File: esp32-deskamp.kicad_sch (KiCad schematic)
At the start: 29 parts, among them J1 INPUT 00, J10 ADDITIONAL GPIO, J2 INPUT 01, J3 MUTE, J4 SLEEP, J5 PRE OUT, J6 LFE OUT, J7 INPUT SELECT, J8 MOTOR, J9 12V IN, K1 INPUT 00, K2 INPUT 01, K3 AMP MUTE, K4 AMP SLEEP, U1 ESP32 D1 MINI, U2 TSR 1-2433, U3 L9110, U4 ULN2003A

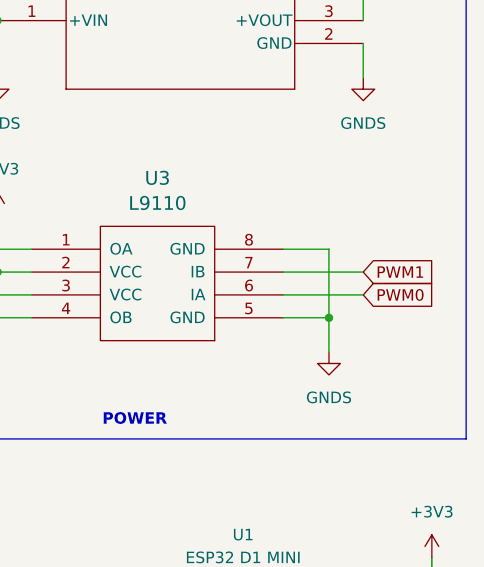
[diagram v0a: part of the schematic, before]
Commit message: Moar routing
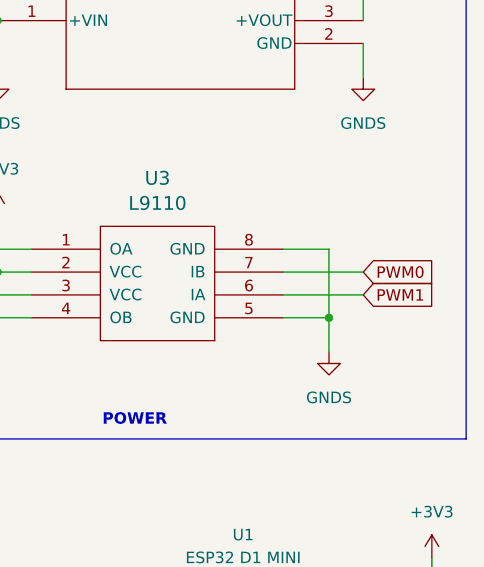
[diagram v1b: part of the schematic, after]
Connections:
- net PWM0: now also U3.7 (IB); no longer U3.6 (IA)
- net PWM1: now also U3.6 (IA); no longer U3.7 (IB)
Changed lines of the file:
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@@
-		)
-	)
-	(global_label "PWM0"
-		(shape input)
-		(at 267.97 59.69 0)
-		(fields_autoplaced yes)
-		(effects
-			(font
-				(size 1.27 1.27)
-			)
-			(justify left)
-		)
-		(property "Intersheetrefs" "${INTERSHEET_REFS}"
-			(at 276.3375 59.69 0)
-			(effects
-				(font
-					(size 1.27 1.27)
-				)
-				(justify left)
-				(hide yes)
-			)
 		)
 	)
@@
 		(property "Intersheetrefs" "${INTERSHEET_REFS}"
 			(at 89.3451 49.53 0)
-			(effects
-				(font
-					(size 1.27 1.27)
-				)
-				(justify left)
-				(hide yes)
-			)
-		)
-	)
-	(global_label "PWM1"
-		(shape input)
-		(at 267.97 57.15 0)
-		(fields_autoplaced yes)
-		(effects
-			(font
-				(size 1.27 1.27)
-			)
-			(justify left)
-		)
-		(property "Intersheetrefs" "${INTERSHEET_REFS}"
-			(at 276.3375 57.15 0)
 			(effects
 				(font
@@
 		)
 	)
+	(global_label "PWM0"
+		(shape input)
+		(at 267.97 57.15 0)
+		(fields_autoplaced yes)
+		(effects
+			(font
+				(size 1.27 1.27)
+			)
+			(justify left)
+		)
+		(property "Intersheetrefs" "${INTERSHEET_REFS}"
+			(at 276.3375 57.15 0)
+			(effects
+				(font
+					(size 1.27 1.27)
+				)
+				(justify left)
+				(hide yes)
+			)
+		)
+	)
 	(global_label "Select0"
 		(shape input)
@@
 				(hide yes)
 			)
+		)
+	)
+	(global_label "PWM1"
+		(shape input)
+		(at 267.97 59.69 0)
+		(fields_autoplaced yes)
+		(effects
+			(font
+				(size 1.27 1.27)
+			)
+			(justify left)
+		)
+		(property "Intersheetrefs" "${INTERSHEET_REFS}"
+			(at 276.3375 59.69 0)
+			(effects
+				(font
+					(size 1.27 1.27)
+				)
+				(justify left)
+				(hide yes)
+			)

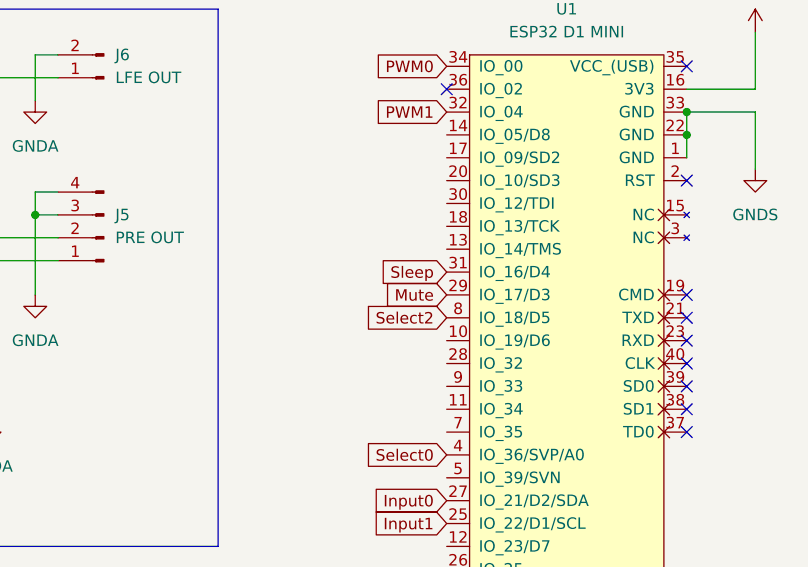
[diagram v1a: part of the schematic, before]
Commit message: Enough for tonight, routed relay control board
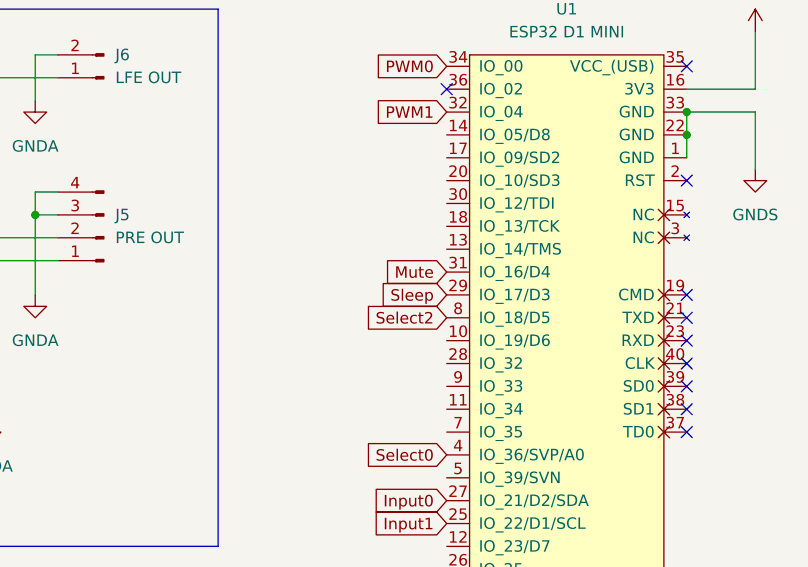
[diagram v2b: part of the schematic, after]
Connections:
- net Mute: now also U1.31 (IO_16/D4); no longer U1.29 (IO_17/D3)
- net Sleep: now also U1.29 (IO_17/D3); no longer U1.31 (IO_16/D4)

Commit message: Moar layout
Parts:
- R7, R8, R9: footprint Resistor_SMD:R_0805_2012Metric_Pad1.20x1.40mm_HandSolder -> Resistor_THT:R_Axial_DIN0204_L3.6mm_D1.6mm_P5.08mm_Horizontal
- U4: footprint Package_SO:SSOP-16_4.4x5.2mm_P0.65mm -> Package_DIP:DIP-16_W7.62mm
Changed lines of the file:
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@@
 			)
 		)
-		(property "Footprint" "Resistor_SMD:R_0805_2012Metric_Pad1.20x1.40mm_HandSolder"
+		(property "Footprint" "Resistor_THT:R_Axial_DIN0204_L3.6mm_D1.6mm_P5.08mm_Horizontal"
 			(at 169.672 35.56 90)
 			(effects
@@
 			)
 		)
-		(property "Footprint" "Resistor_SMD:R_0805_2012Metric_Pad1.20x1.40mm_HandSolder"
+		(property "Footprint" "Resistor_THT:R_Axial_DIN0204_L3.6mm_D1.6mm_P5.08mm_Horizontal"
 			(at 151.892 35.56 90)
 			(effects
@@
 			)
 		)
-		(property "Footprint" "Package_SO:SSOP-16_4.4x5.2mm_P0.65mm"
+		(property "Footprint" "Package_DIP:DIP-16_W7.62mm"
 			(at 111.76 118.11 0)
 			(effects
@@
 			)
 		)
-		(property "Footprint" "Resistor_SMD:R_0805_2012Metric_Pad1.20x1.40mm_HandSolder"
+		(property "Footprint" "Resistor_THT:R_Axial_DIN0204_L3.6mm_D1.6mm_P5.08mm_Horizontal"
 			(at 160.782 35.56 90)
 			(effects
